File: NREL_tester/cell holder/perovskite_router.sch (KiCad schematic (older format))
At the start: 5 parts, among them J1 Conn_01x10_Male, J2 Conn_01x10_Male, U1 Perovskite_CP_6_Cell, U2 MCP9808_MSOP

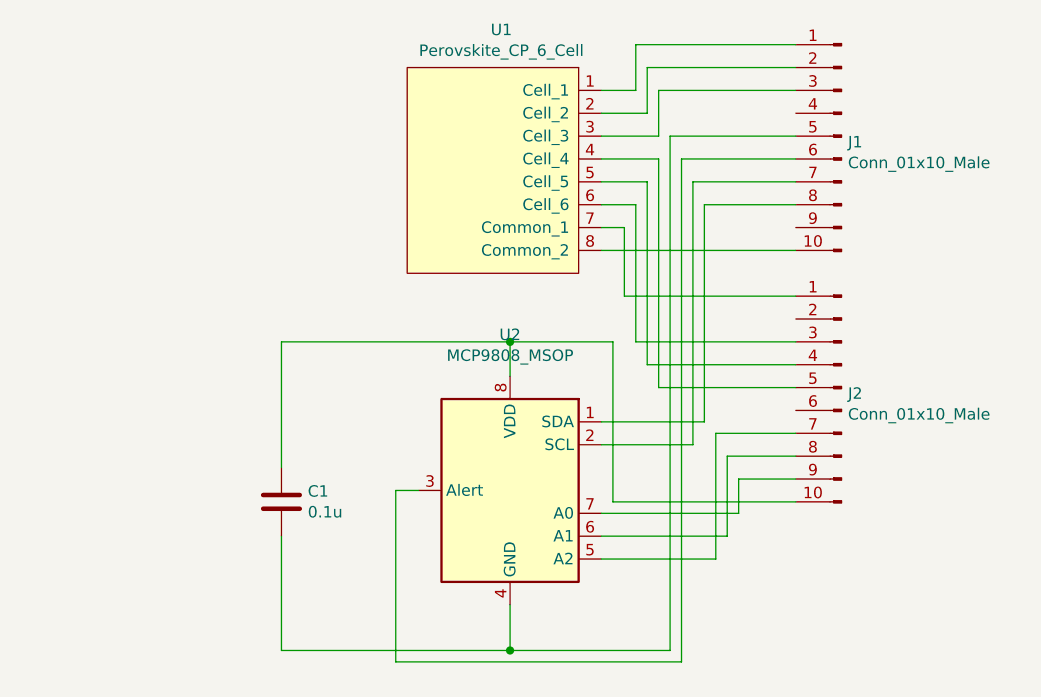
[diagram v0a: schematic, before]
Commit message: Review contact board
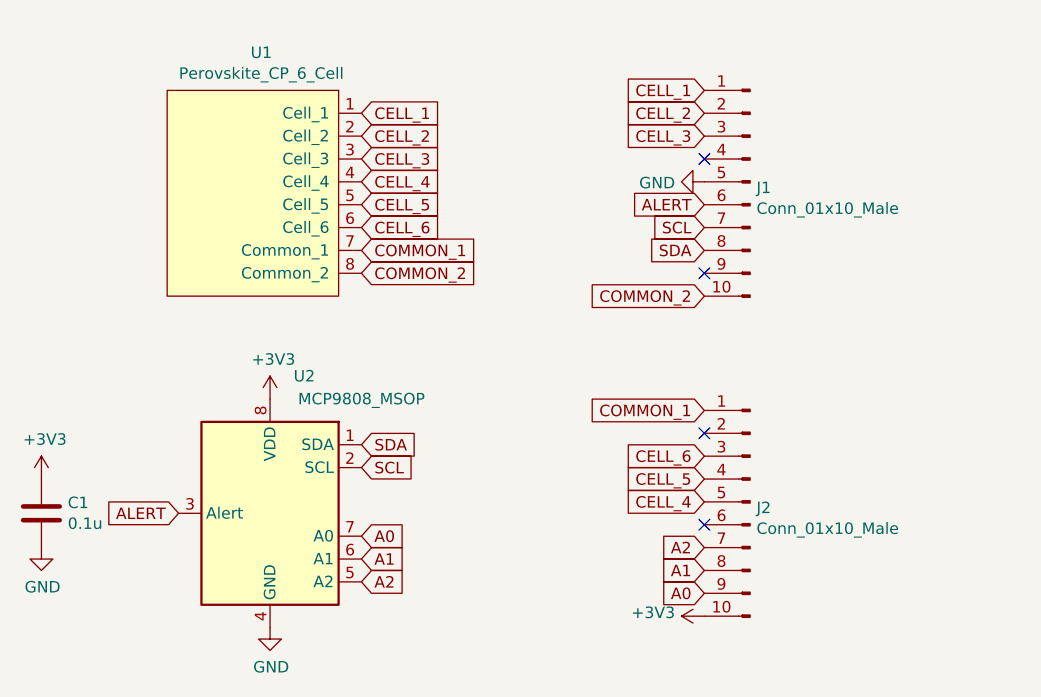
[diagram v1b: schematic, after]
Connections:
- net CELL_1: now reaches J1.1 (Pin_1), U1.1 (Cell_1)
- net CELL_2: now reaches J1.2 (Pin_2), U1.2 (Cell_2)
- net CELL_3: now reaches J1.3 (Pin_3), U1.3 (Cell_3)
- net CELL_4: now reaches J2.5 (Pin_5), U1.4 (Cell_4)
- net CELL_5: now reaches J2.4 (Pin_4), U1.5 (Cell_5)
- net CELL_6: now reaches J2.3 (Pin_3), U1.6 (Cell_6)
- net COMMON_1: now reaches J2.1 (Pin_1), U1.7 (Common_1)
- net COMMON_2: now reaches J1.10 (Pin_10), U1.8 (Common_2)
- net SDA: now reaches J1.8 (Pin_8), U2.1 (SDA)
- net SCL: now reaches J1.7 (Pin_7), U2.2 (SCL)
- net ALERT: now reaches J1.6 (Pin_6), U2.3 (Alert)
- net GND: now reaches C1.2, J1.5 (Pin_5), U2.4 (GND)
- net A2: now reaches J2.7 (Pin_7), U2.5 (A2)
- net A1: now reaches J2.8 (Pin_8), U2.6 (A1)
- net A0: now reaches J2.9 (Pin_9), U2.7 (A0)
- net +3V3: now reaches C1.1, J2.10 (Pin_10), U2.8 (VDD)
- no-connect marks 0 -> 4
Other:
- moved on the sheet: C1, J1, J2, U1, U2
